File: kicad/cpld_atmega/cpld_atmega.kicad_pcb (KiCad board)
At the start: 2 copper layers, 82.5 x 52.7 mm, 35 parts, among them CON1 AVR-ISP-6, J1 PWR, J10 FB 4, J2 ADC, J3 Port B, J4 PORT D, J5 Port C, J6 FB 1, J7 FB 2, J8 JTAG, J9 FB 3, SW1 SW_Push, SW2 PWR, U1 LM1117-3.3, U2 ATMEGA168A-AU, U3 XC9572XL-VQFP44, Y1 12Mhz

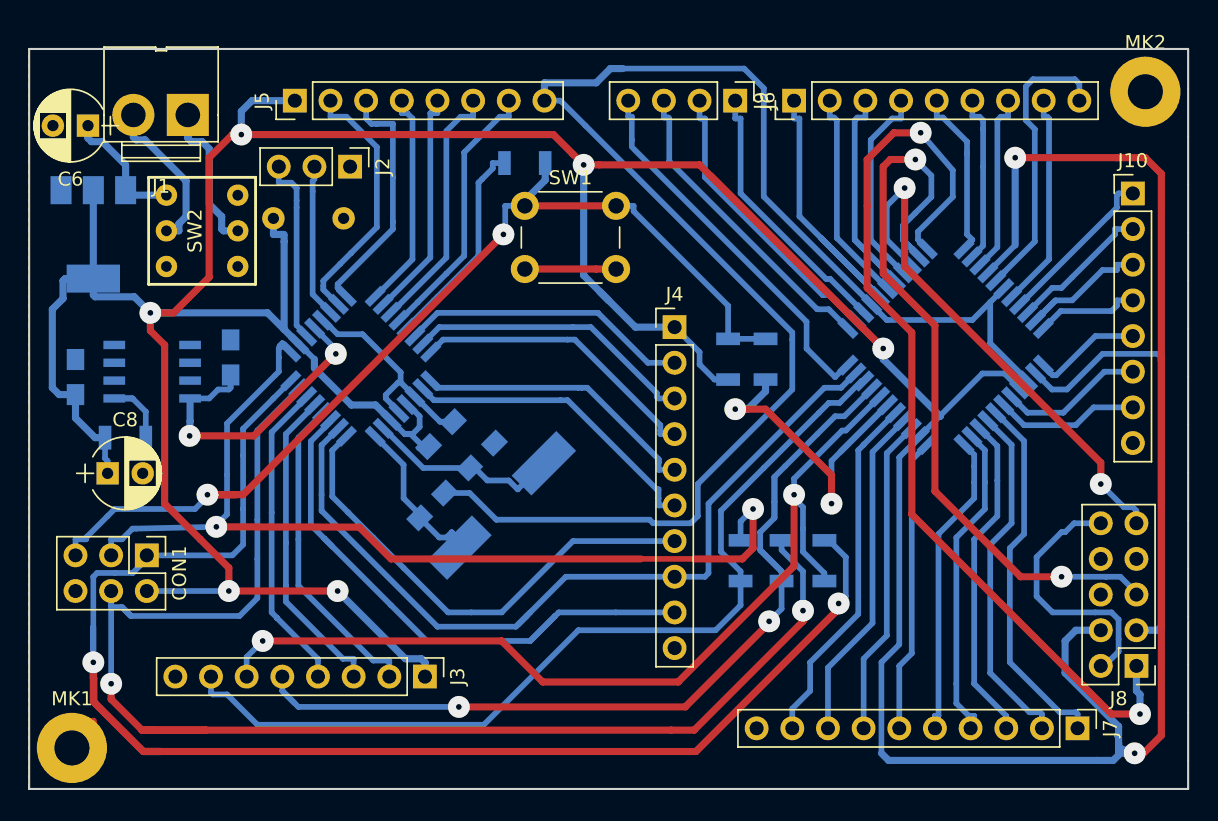
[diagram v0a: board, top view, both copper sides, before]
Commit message: version 0.1
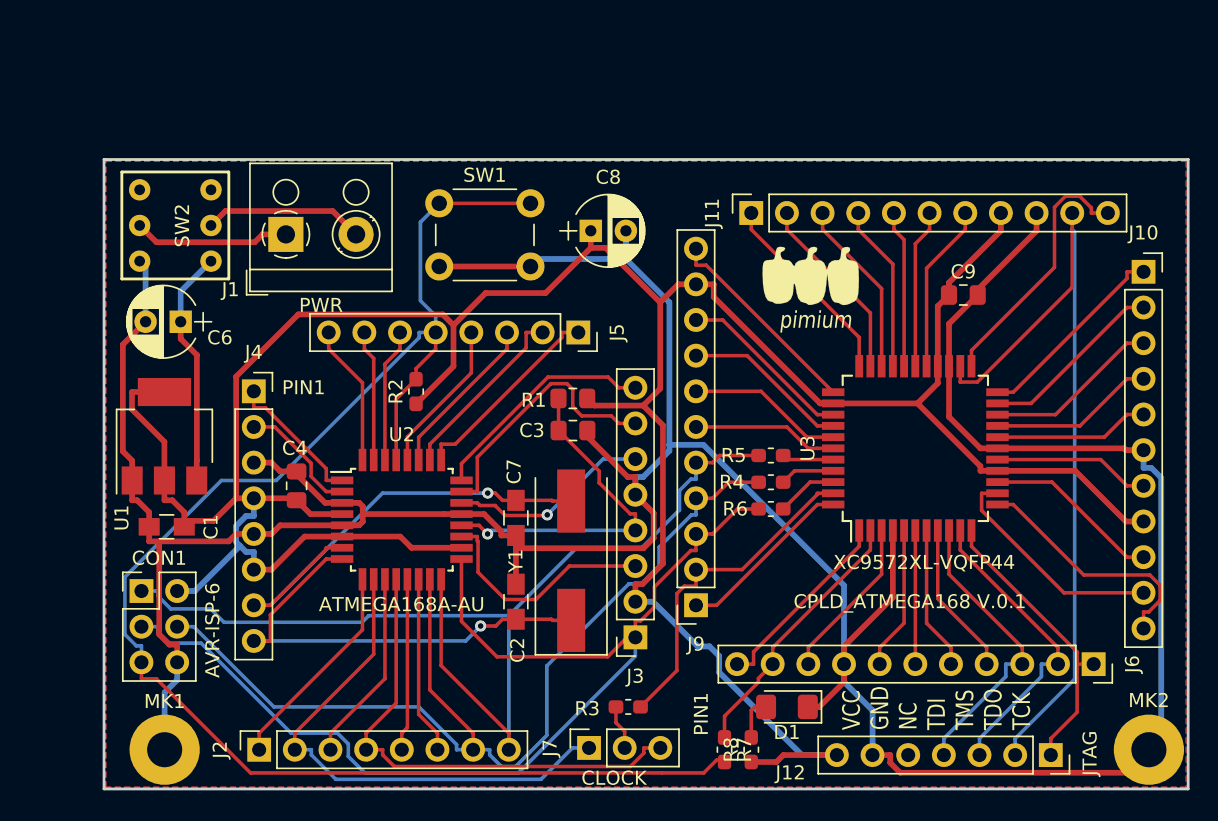
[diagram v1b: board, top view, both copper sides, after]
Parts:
- removed C5: 100n, Capacitors_THT:C_Disc_D4.3mm_W1.9mm_P5.00mm
- removed J8: JTAG, Pin_Headers:Pin_Header_Straight_2x05_Pitch2.54mm
- added C3: 100n, Capacitor_SMD:C_0805_2012Metric_Pad1.15x1.40mm_HandSolder, F.Cu at (61.6, 71.6)
- added G***: LOGO, custom_logo:pimium_paprika_7mm, F.Cu at (78.5, 61.8)
- added J11: Conn_01x11, Connector_PinSocket_2.54mm:PinSocket_1x11_P2.54mm_Vertical, F.Cu at (74.3, 56.1)
- added J12: JTAG, Connector_PinSocket_2.54mm:PinSocket_1x07_P2.54mm_Vertical, F.Cu at (95.6, 94.7)
- added R8: 470, Resistor_SMD:R_0603_1608Metric_Pad1.05x0.95mm_HandSolder, F.Cu at (74.3, 94.4)
- C1, C2, C7, U1, U2, Y1: moved to F.Cu
- C4, C9: footprint Capacitors_SMD:C_0805_HandSoldering -> Capacitor_SMD:C_0805_2012Metric_Pad1.15x1.40mm_HandSolder; moved to F.Cu
- D1: value TL431D -> LED; footprint Housings_SOIC:SOIC-8_3.9x4.9mm_Pitch1.27mm -> LED_SMD:LED_1206_3216Metric_Pad1.42x1.75mm_HandSolder; moved to F.Cu
- J1: footprint Connectors:JWT_Vertical_A3963-RM3.96mm-2 -> TerminalBlock_RND:TerminalBlock_RND_205-00001_1x02_P5.00mm_Horizontal
- J10: value FB 4 -> Conn_01x11; footprint Pin_Headers:Pin_Header_Straight_1x08_Pitch2.54mm -> Connector_PinSocket_2.54mm:PinSocket_1x11_P2.54mm_Vertical
- J2: value ADC -> Conn_01x08_Male; footprint Pin_Headers:Pin_Header_Straight_1x03_Pitch2.54mm -> Connector_PinSocket_2.54mm:PinSocket_1x08_P2.54mm_Vertical
- J3: value Port B -> Conn_01x08_Male; footprint Pin_Headers:Pin_Header_Straight_1x08_Pitch2.54mm -> Connector_PinSocket_2.54mm:PinSocket_1x08_P2.54mm_Vertical
- J4: value PORT D -> Conn_01x08_Male; footprint Pin_Headers:Pin_Header_Straight_1x10_Pitch2.54mm -> Connector_PinSocket_2.54mm:PinSocket_1x08_P2.54mm_Vertical
- J5: value Port C -> Conn_01x08_Male; footprint Pin_Headers:Pin_Header_Straight_1x08_Pitch2.54mm -> Connector_PinSocket_2.54mm:PinSocket_1x08_P2.54mm_Vertical
- J6: value FB 1 -> Conn_01x11; footprint Pin_Headers:Pin_Header_Straight_1x04_Pitch2.54mm -> Connector_PinSocket_2.54mm:PinSocket_1x11_P2.54mm_Vertical
- J7: value FB 2 -> CLOCK; footprint Pin_Headers:Pin_Header_Straight_1x10_Pitch2.54mm -> Connector_PinSocket_2.54mm:PinSocket_1x03_P2.54mm_Vertical
- J9: value FB 3 -> Conn_01x11; footprint Pin_Headers:Pin_Header_Straight_1x09_Pitch2.54mm -> Connector_PinSocket_2.54mm:PinSocket_1x11_P2.54mm_Vertical
- R1: value 1k -> 0; footprint Resistors_SMD:R_1206 -> Resistor_SMD:R_0805_2012Metric_Pad1.15x1.40mm_HandSolder; moved to F.Cu
- R2: value 4k7 -> 10K; footprint Resistors_SMD:R_1206 -> Resistor_SMD:R_0603_1608Metric_Pad1.05x0.95mm_HandSolder; moved to F.Cu
- R3: value 4k7 -> 1k; footprint Resistors_SMD:R_1206 -> Resistor_SMD:R_0603_1608Metric_Pad1.05x0.95mm_HandSolder; moved to F.Cu
- R4, R5, R6: footprint Resistors_SMD:R_1206 -> Resistor_SMD:R_0603_1608Metric_Pad1.05x0.95mm_HandSolder; moved to F.Cu
- R7: value 4k7 -> 1K; footprint Resistors_SMD:R_1206 -> Resistor_SMD:R_0603_1608Metric_Pad1.05x0.95mm_HandSolder; moved to F.Cu
- U3: footprint Housings_QFP:LQFP-44_10x10mm_Pitch0.8mm -> Package_QFP:LQFP-44_10x10mm_P0.8mm; moved to F.Cu
- moved C9 63.5 mm to (89.4, 62.0), turned to 0 degrees
- moved D1 51.1 mm to (76.8, 91.3), turned to 180 degrees
- moved J6 47.6 mm to (98.7, 88.3)
- moved MK2 46.9 mm to (102.6, 94.4)
- moved J2 42.0 mm to (39.2, 94.4), turned to 90 degrees
- moved R3 39.4 mm to (65.5, 91.3), turned to 0 degrees
- moved C8 38.5 mm to (62.9, 57.4)
- moved J9 36.6 mm to (70.4, 84.1), turned to 180 degrees
- moved J7 34.8 mm to (62.7, 94.2), turned to 90 degrees
- moved R1 32.0 mm to (61.6, 69.3), turned to 180 degrees
- moved J4 30.3 mm to (38.9, 68.8)
- moved R7 28.0 mm to (72.4, 94.4), turned to 270 degrees
- moved J5 26.1 mm to (62.0, 64.6), turned to 270 degrees
- moved R2 22.3 mm to (50.4, 68.8)
- moved C6 15.5 mm to (33.7, 63.9)
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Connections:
- C1 pad 1: +2V5 -> VCC
- C2 pad 1: /XTAL1 -> /P8
- C7 pad 1: /XTAL2 -> /P7
- CON1 pad 3: /SCK -> /P17
- D1 pad 1: Net-(D1-Pad1) -> GND
- D1 pad 2: GND -> Net-(D1-Pad2)
- J10 pad 6: Net-(J10-Pad6) -> GND
- J10 pad 8: GND -> VCC
- J2 pad 1: GND -> /P9
- J2 pad 2: Net-(J2-Pad2) -> /P10
- J2 pad 3: Net-(J2-Pad3) -> /P11
- J3 pad 1: VCC -> /P17
- J3 pad 2: Net-(J3-Pad2) -> VCC
- J3 pad 3: Net-(J3-Pad3) -> /P19
- J3 pad 4: Net-(J3-Pad4) -> /P20
- J3 pad 5: /MOSI_ -> GND
- J3 pad 6: /MISO_ -> /P22
- J3 pad 7: /SCK_ -> /P23
- J3 pad 8: GND -> /P24
- J4 pad 1: VCC -> /P1
- J4 pad 2: Net-(J4-Pad2) -> /P2
- J4 pad 3: Net-(J4-Pad3) -> GND
- J4 pad 4: Net-(J4-Pad4) -> VCC
- J4 pad 5: Net-(J4-Pad5) -> GND
- J4 pad 6: Net-(J4-Pad6) -> VCC
- J4 pad 7: Net-(J4-Pad7) -> /P7
- J4 pad 8: /CCLK -> /P8
- J5 pad 1: VCC -> /P25
- J5 pad 2: /PC0 -> /P26
- J5 pad 3: /PC1 -> /P27
- J5 pad 4: /PC2 -> /P28
- J5 pad 5: /PC3 -> /RESET
- J5 pad 6: /PC4 -> /P30
- J5 pad 7: /PC5 -> /P31
- J5 pad 8: GND -> /P32
- J6 pad 1: Net-(J6-Pad1) -> /TCK
- J6 pad 2: Net-(J6-Pad2) -> /TMS
- J6 pad 3: Net-(J6-Pad3) -> /TDI
- J7 pad 1: Net-(J7-Pad1) -> /P10
- J7 pad 3: Net-(J7-Pad3) -> /CCLK
- J9 pad 3: Net-(J9-Pad3) -> /P17
- J9 pad 4: Net-(J9-Pad4) -> /MOSI
- J9 pad 5: Net-(J9-Pad5) -> /MISO
- R1 pad 2: Net-(D1-Pad1) -> /P20
- R3 pad 1: /RESET -> Net-(J7-Pad2)
- R3 pad 2: Net-(R3-Pad2) -> Net-(J9-Pad2)
- R4 pad 1: /MOSI_ -> Net-(R4-Pad1)
- R5 pad 1: /MISO_ -> Net-(R5-Pad1)
- R6 pad 1: /SCK_ -> Net-(R6-Pad1)
- R6 pad 2: /SCK -> /P17
- R7 pad 1: Net-(R7-Pad1) -> Net-(J6-Pad10)
- U2 pad 1: Net-(J4-Pad5) -> /P1
- U2 pad 10: /CCLK -> /P10
- U2 pad 11: Net-(J4-Pad9) -> /P11
- U2 pad 12: Net-(J3-Pad2) -> /CCLK
- U2 pad 13: Net-(J3-Pad3) -> /P13
- U2 pad 14: Net-(J3-Pad4) -> /P14
- U2 pad 17: /SCK -> /P17
- U2 pad 19: Net-(J2-Pad3) -> /P19
- U2 pad 2: Net-(J4-Pad6) -> /P2
- U2 pad 20: +2V5 -> /P20
- U2 pad 22: Net-(J2-Pad2) -> /P22
- U2 pad 23: /PC0 -> /P23
- U2 pad 24: /PC1 -> /P24
- U2 pad 25: /PC2 -> /P25
- U2 pad 26: /PC3 -> /P26
- U2 pad 27: /PC4 -> /P27
- U2 pad 28: /PC5 -> /P28
- U2 pad 29: Net-(R3-Pad2) -> /RESET
- U2 pad 30: Net-(J4-Pad2) -> /P30
- U2 pad 31: Net-(J4-Pad3) -> /P31
- U2 pad 32: Net-(J4-Pad4) -> /P32
- U2 pad 7: /XTAL2 -> /P7
- U2 pad 8: /XTAL1 -> /P8
- U2 pad 9: Net-(J4-Pad7) -> /P9
- U3 pad 1: Net-(J6-Pad3) -> Net-(J6-Pad11)
- U3 pad 12: Net-(J9-Pad5) -> Net-(J10-Pad11)
- U3 pad 13: Net-(J9-Pad6) -> Net-(J10-Pad10)
- U3 pad 14: Net-(J9-Pad7) -> Net-(J10-Pad9)
- U3 pad 16: Net-(J9-Pad9) -> Net-(J10-Pad7)
- U3 pad 18: Net-(J9-Pad8) -> Net-(J10-Pad5)
- U3 pad 19: Net-(J10-Pad1) -> Net-(J10-Pad4)
- U3 pad 2: Net-(J6-Pad2) -> Net-(J6-Pad10)
- U3 pad 20: Net-(J10-Pad2) -> Net-(J10-Pad3)
- U3 pad 21: Net-(J10-Pad3) -> Net-(J10-Pad2)
- U3 pad 22: Net-(J10-Pad4) -> Net-(J10-Pad1)
- U3 pad 23: Net-(J10-Pad5) -> Net-(J11-Pad11)
- U3 pad 27: Net-(J10-Pad6) -> Net-(J11-Pad7)
- U3 pad 28: Net-(J10-Pad7) -> Net-(J11-Pad6)
- U3 pad 29: Net-(J7-Pad1) -> Net-(J11-Pad5)
- U3 pad 3: Net-(J6-Pad1) -> Net-(J6-Pad9)
- U3 pad 30: Net-(J7-Pad2) -> Net-(J11-Pad4)
- U3 pad 31: Net-(J7-Pad3) -> Net-(J11-Pad3)
- U3 pad 32: Net-(J7-Pad4) -> Net-(J11-Pad2)
- U3 pad 33: Net-(J7-Pad5) -> Net-(J11-Pad1)
- U3 pad 34: Net-(J7-Pad6) -> Net-(J9-Pad11)
- U3 pad 36: Net-(J7-Pad7) -> Net-(J9-Pad9)
- U3 pad 37: Net-(J7-Pad8) -> Net-(J9-Pad8)
- U3 pad 38: Net-(J7-Pad9) -> Net-(J9-Pad7)
- U3 pad 39: Net-(R7-Pad1) -> Net-(J9-Pad6)
- U3 pad 40: /MISO_ -> Net-(R5-Pad1)
- U3 pad 41: /MOSI_ -> Net-(R4-Pad1)
- U3 pad 42: /SCK_ -> Net-(R6-Pad1)
- U3 pad 43: /CCLK -> Net-(J9-Pad2)
- U3 pad 44: Net-(J6-Pad4) -> Net-(J9-Pad1)
- U3 pad 5: Net-(J9-Pad1) -> Net-(J6-Pad7)
- U3 pad 6: Net-(J9-Pad2) -> Net-(J6-Pad6)
- U3 pad 7: Net-(J9-Pad3) -> Net-(J6-Pad5)
- U3 pad 8: Net-(J9-Pad4) -> Net-(J6-Pad4)
- Y1 pad 1: /XTAL1 -> /P8
- Y1 pad 2: /XTAL2 -> /P7
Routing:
- net VCC: track 369.6 -> 219.9 mm, vias 8 -> 0
- net GND: track 156.1 -> 254.8 mm
- net /P17: track 0.00 -> 78.5 mm
- net /SCK: track 75.3 -> 0.00 mm, vias 2 -> 0
- net /MISO_: track 67.3 -> 0.00 mm, vias 2 -> 0
- net /MOSI_: track 66.3 -> 0.00 mm, vias 2 -> 0
- net /SCK_: track 64.7 -> 0.00 mm
- net /TCK: track 73.6 -> 21.1 mm, vias 2 -> 0
- net Net-(J4-Pad9): track 41.6 -> 0.00 mm
- net /MISO: track 113.5 -> 75.2 mm, vias 2 -> 0
- net /P10: track 0.00 -> 37.4 mm
- net /RESET: track 73.3 -> 109.2 mm, vias 2 -> 0
- net Net-(J4-Pad7): track 34.6 -> 0.00 mm
- net /P7: track 0.00 -> 34.2 mm, vias 0 -> 1
- net /TMS: track 55.7 -> 21.9 mm, vias 2 -> 0
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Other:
- board size 82.5 x 52.7 mm -> 77.2 x 44.8 mm
- net class Default: clearance 0.2 -> 0.20066; trace_width 0.25 -> 0.254
- net class Signal: clearance 0.2 -> 0.20828
- rule trace_clearance: 0.2 -> 0.20066
- board text added: "CPLD_ATMEGA168 V.0.1"
- board text added: "PIN1"
- board text added: "VCC GND NC TDI TMS TDO TCK"
- board text removed: "GND"
- board text removed: "NC"
- board text removed: "P1"
- board text removed: "P12"
- board text removed: "P13"
- board text removed: "P14"
- board text removed: "P16"
- board text removed: "P18"
- board text removed: "P19"
- board text removed: "P2"
- board text removed: "P20"
- board text removed: "P21"
- board text removed: "P22"
- board text removed: "P23"
- board text removed: "P27"
- board text removed: "P28"
- board text removed: "P29"
- board text removed: "P3"
- board text removed: "P30"
- board text removed: "P33"
- board text removed: "P34"
- board text removed: "P36"
- board text removed: "P37"
- board text removed: "P38"
- board text removed: "P39 = RESET P40 = MISO P41 = MOSI P42 = SCK P43 = CCLK"
- board text removed: "P43"
- board text removed: "P44"
- board text removed: "P5"
- board text removed: "P6"
- board text removed: "P7"
- board text removed: "P8"
- board text removed: "PB0"
- board text removed: "PB1"
- board text removed: "PB2"
- board text removed: "PB3/MOSI"
- board text removed: "PB4/MISO"
- board text removed: "PB5/SCK"
- board text removed: "PC0"
- board text removed: "PC1"
- board text removed: "PC2"
- board text removed: "PC3"
- board text removed: "PC4"
- board text removed: "PC5"
- board text removed: "PC6"
- board text removed: "PD1"
- board text removed: "PD2"
- board text removed: "PD3"
- board text removed: "PD4"
- board text removed: "PD5"
- board text removed: "PD6"
- board text removed: "PD7"
- board text removed: "PWR"
- board text removed: "RESET"
- board text removed: "TCK"
- board text removed: "TDI"
- board text removed: "TDO"
- board text removed: "TMS"
- board text removed: "VCC"
